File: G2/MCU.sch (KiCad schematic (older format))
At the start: 2 parts

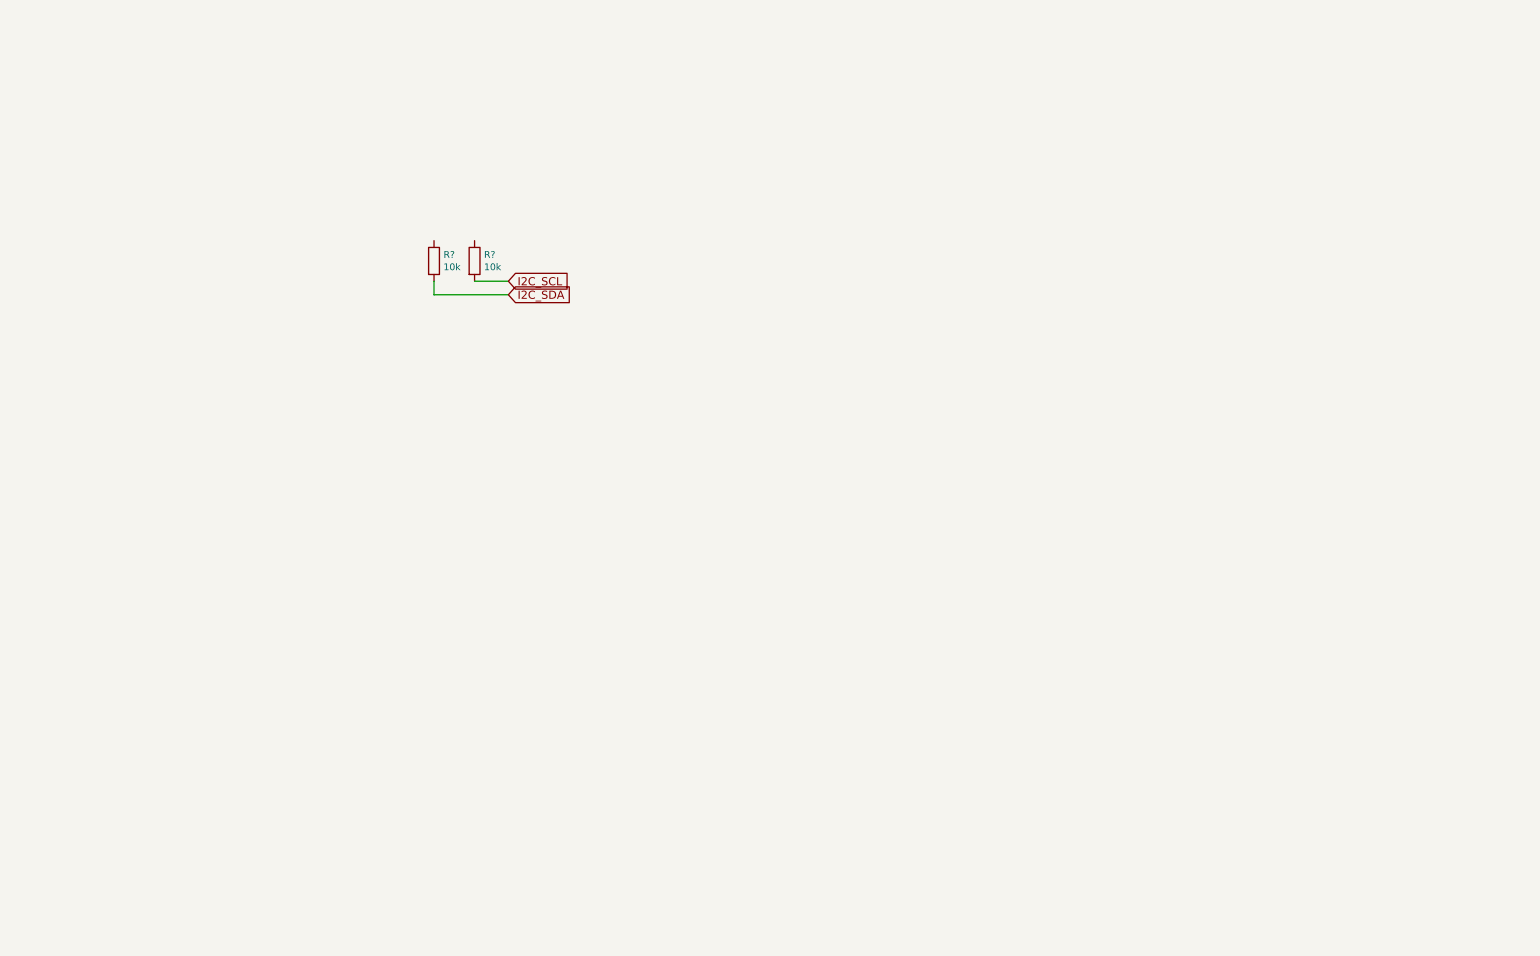
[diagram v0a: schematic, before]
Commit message: Most things connected to MCU
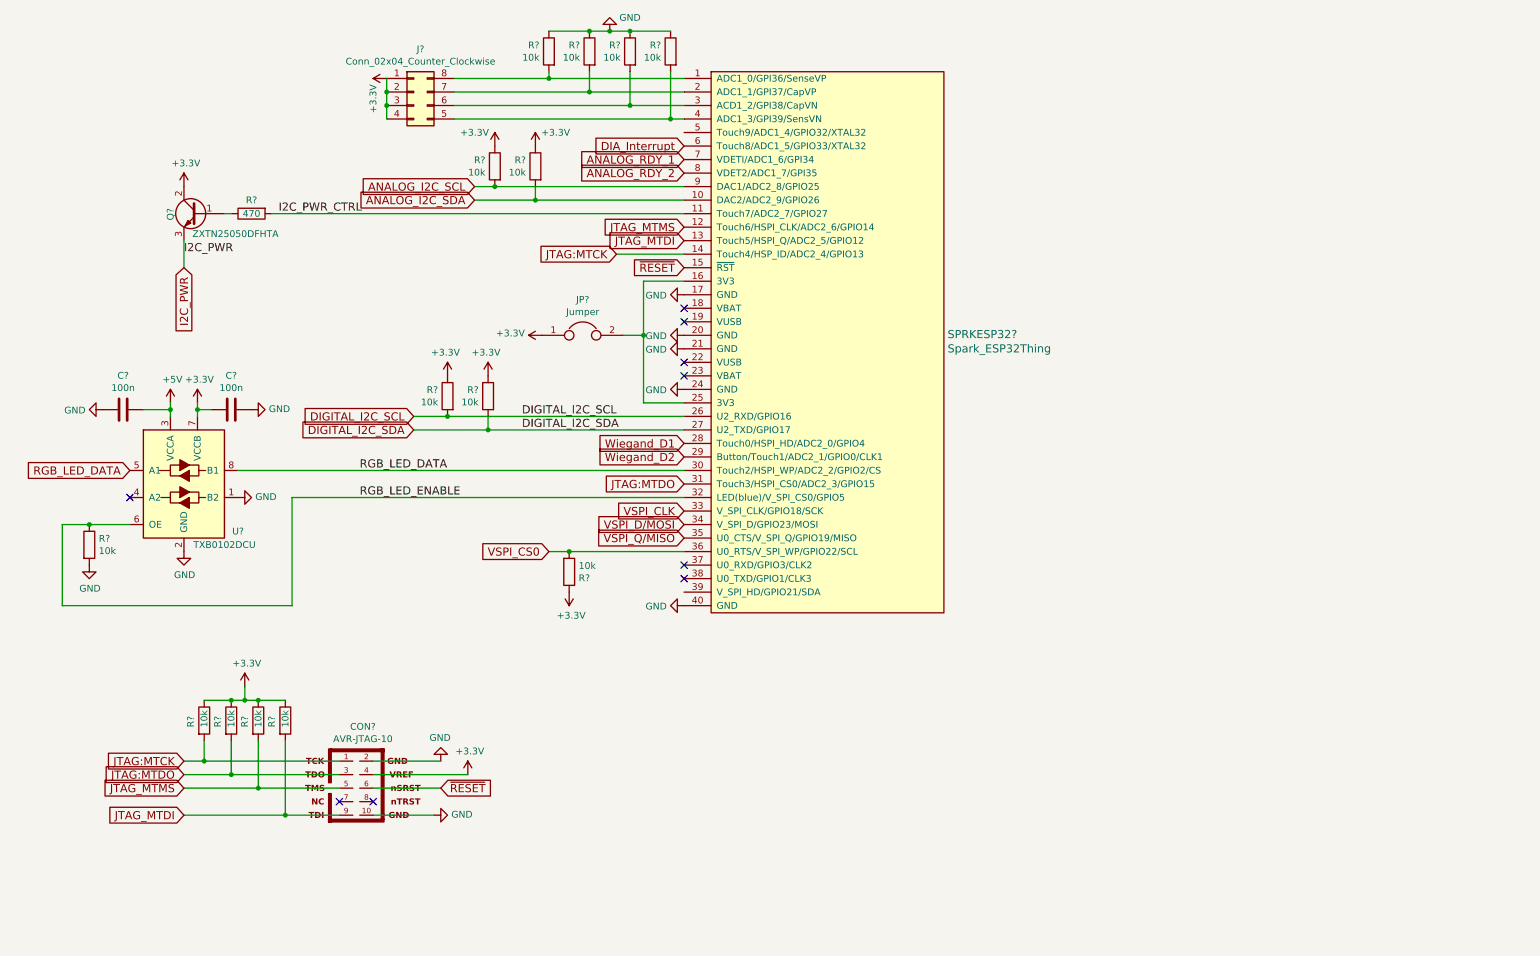
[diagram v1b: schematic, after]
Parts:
- added C? (x2): 100n, Capacitors_SMD:C_0805, symbol C
- added CON?: AVR-JTAG-10, Pin_Headers:Pin_Header_Straight_2x05_Pitch2.54mm, symbol AVR-JTAG-10
- added J?: Conn_02x04_Counter_Clockwise, Housings_DIP:DIP-8_W9.53mm_SMD, symbol Conn_02x04_Counter_Clockwise
- added JP?: Jumper, Pin_Headers:Pin_Header_Straight_1x02_Pitch2.54mm, symbol Jumper
- added Q?: ZXTN25050DFHTA, TO_SOT_Packages_SMD:SOT-23, symbol Q_NPN_BCE
- added R? (x11): 10k, Resistors_SMD:R_0805, symbol R
- added R?: 10k, symbol R
- added R?: 470, Resistors_SMD:R_0805, symbol R
- added SPRKESP32?: Spark_ESP32Thing, symbol Spark_ESP32Thing
- added U?: TXB0102DCU, Housings_SSOP:VSSOP-8_2.4x2.1mm_Pitch0.5mm, symbol TXB0102DCU
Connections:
- net +3V3: now reaches R?.1
- net +3V3: now also R?.1, C?.2, CON?.4, J?.1 (Pin_1), J?.2 (Pin_2), J?.3 (Pin_3), J?.4 (Pin_4), JP?.1, Q?.2 (C), R?.1, R?.1, R?.1, R?.1, R?.1, R?.1, R?.1, U?.7 (VCCB)
- net I2C_SCL renamed DIGITAL_I2C_SCL
- net DIGITAL_I2C_SCL: now also SPRKESP32?.26 (U2_RXD/GPIO16)
- net I2C_SDA renamed DIGITAL_I2C_SDA
- net DIGITAL_I2C_SDA: now also SPRKESP32?.27 (U2_TXD/GPIO17)
- new net: J?.8 (Pin_8), R?.2, SPRKESP32?.1 (ADC1_0/GPI36/SenseVP)
- new net: JP?.2, SPRKESP32?.16 (3V3), SPRKESP32?.25 (3V3)
- new net: J?.7 (Pin_7), R?.2, SPRKESP32?.2 (ADC1_1/GPI37/CapVP)
- new net: J?.6 (Pin_6), R?.2, SPRKESP32?.3 (ACD1_2/GPI38/CapVN)
- new net: J?.5 (Pin_5), R?.2, SPRKESP32?.4 (ADC1_3/GPI39/SensVN)
- new net: Q?.1 (B), R?.1
- new net +5V: C?.1, U?.3 (VCCA)
- new net ANALOG_I2C_SCL: R?.2, SPRKESP32?.9 (DAC1/ADC2_8/GPIO25)
- new net ANALOG_I2C_SDA: R?.2, SPRKESP32?.10 (DAC2/ADC2_9/GPIO26)
- new net ANALOG_RDY_1: SPRKESP32?.7 (VDETI/ADC1_6/GPI34)
- new net ANALOG_RDY_2: SPRKESP32?.8 (VDET2/ADC1_7/GPI35)
- new net DIA_Interrupt: SPRKESP32?.6 (Touch8/ADC1_5/GPIO33/XTAL32)
- new net GND: C?.1, C?.2, CON?.10, CON?.2, R?.1, R?.1, R?.1, R?.1, R?.2, SPRKESP32?.17 (GND), SPRKESP32?.20 (GND), SPRKESP32?.21 (GND), SPRKESP32?.24 (GND), SPRKESP32?.40 (GND), U?.1 (B2), U?.2 (GND)
- new net I2C_PWR: Q?.3 (E)
- new net I2C_PWR_CTRL: R?.2, SPRKESP32?.11 (Touch7/ADC2_7/GPIO27)
- new net JTAG:MTCK: CON?.1, R?.2, SPRKESP32?.14 (Touch4/HSP_ID/ADC2_4/GPIO13)
- new net JTAG:MTDO: CON?.3, R?.2, SPRKESP32?.31 (Touch3/HSPI_CS0/ADC2_3/GPIO15)
- new net JTAG_MTDI: CON?.9, R?.2, SPRKESP32?.13 (Touch5/HSPI_Q/ADC2_5/GPIO12)
- new net JTAG_MTMS: CON?.5, R?.2, SPRKESP32?.12 (Touch6/HSPI_CLK/ADC2_6/GPIO14)
- new net RGB_LED_DATA: SPRKESP32?.30 (Touch2/HSPI_WP/ADC2_2/GPIO2/CS), U?.5 (A1), U?.8 (B1)
- new net RGB_LED_ENABLE: R?.1, SPRKESP32?.32 (LED(blue)/V_SPI_CS0/GPIO5), U?.6 (OE)
- new net VSPI_CLK: SPRKESP32?.33 (V_SPI_CLK/GPIO18/SCK)
- new net VSPI_CS0: R?.2, SPRKESP32?.36 (U0_RTS/V_SPI_WP/GPIO22/SCL)
- new net VSPI_D/MOSI: SPRKESP32?.34 (V_SPI_D/GPIO23/MOSI)
- new net VSPI_Q/MISO: SPRKESP32?.35 (U0_CTS/V_SPI_Q/GPIO19/MISO)
- new net Wiegand_D1: SPRKESP32?.28 (Touch0/HSPI_HD/ADC2_0/GPIO4)
- new net Wiegand_D2: SPRKESP32?.29 (Button/Touch1/ADC2_1/GPIO0/CLK1)
- new net ~RESET: CON?.6, SPRKESP32?.15 (~RST)
- no-connect marks 0 -> 9
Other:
- moved on the sheet: R?

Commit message: Begun layout.
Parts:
- removed C? (x2): 100n, Capacitors_SMD:C_0805, symbol C
- removed Q?: ZXTN25050DFHTA, TO_SOT_Packages_SMD:SOT-23, symbol Q_NPN_BCE
- removed R?: 10k, symbol R
- removed R?: 470, Resistors_SMD:R_0805, symbol R
- removed U?: TXB0102DCU, Housings_SSOP:VSSOP-8_2.4x2.1mm_Pitch0.5mm, symbol TXB0102DCU
- added C401, C402: 100n, Capacitors_SMD:C_0805, symbol C
- added J401: Conn_02x06_Counter_Clockwise, Pin_Headers:Pin_Header_Straight_2x06_Pitch2.54mm, symbol Conn_02x06_Counter_Clockwise
- added J402: Conn_02x08_Counter_Clockwise, Pin_Headers:Pin_Header_Straight_2x08_Pitch2.54mm, symbol Conn_02x08_Counter_Clockwise
- added R405: 10k, Resistors_SMD:R_0805, symbol R
- added U401: TXB0102DCU, Housings_SSOP:VSSOP-8_2.4x2.1mm_Pitch0.5mm, symbol TXB0102DCU
- SPRKESP32401: renamed from SPRKESP32?; footprint (none) -> spark_esp32thing:Sparkfun_ESP32Thing
- gave numbers to parts that had none: 16
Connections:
- net labels added: +3V3_C, +5V_C, BELL_CTRL, GND_C, LEVEL_SHIFTER_ENABLE, RGB_LED_DATA_CTRL
- net labels removed: +3.3V, +5V, GND, I2C_PWR, RGB_LED_DATA, RGB_LED_ENABLE
- wire segments 74 -> 100
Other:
- note added: "To Status"
- note added: "To backplane"
- moved on the sheet: CON401, J403, JP401, R401, R402, R403, R404, R406, R407, R408, R409, R410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

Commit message: Layout of IO board completed, except bell transistor.
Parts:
- removed J402: Conn_02x08_Counter_Clockwise, Pin_Headers:Pin_Header_Straight_2x08_Pitch2.54mm, symbol Conn_02x08_Counter_Clockwise
- added J402: Conn_02x08_Odd_Even, Pin_Headers:Pin_Header_Straight_2x08_Pitch2.54mm, symbol Conn_02x08_Odd_Even
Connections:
- wire segments 100 -> 106
